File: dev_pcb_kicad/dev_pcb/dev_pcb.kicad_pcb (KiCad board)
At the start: 2 copper layers, 33 x 37.5 mm, 11 parts, among them U2 XIAO-ESP32-S3-DIP

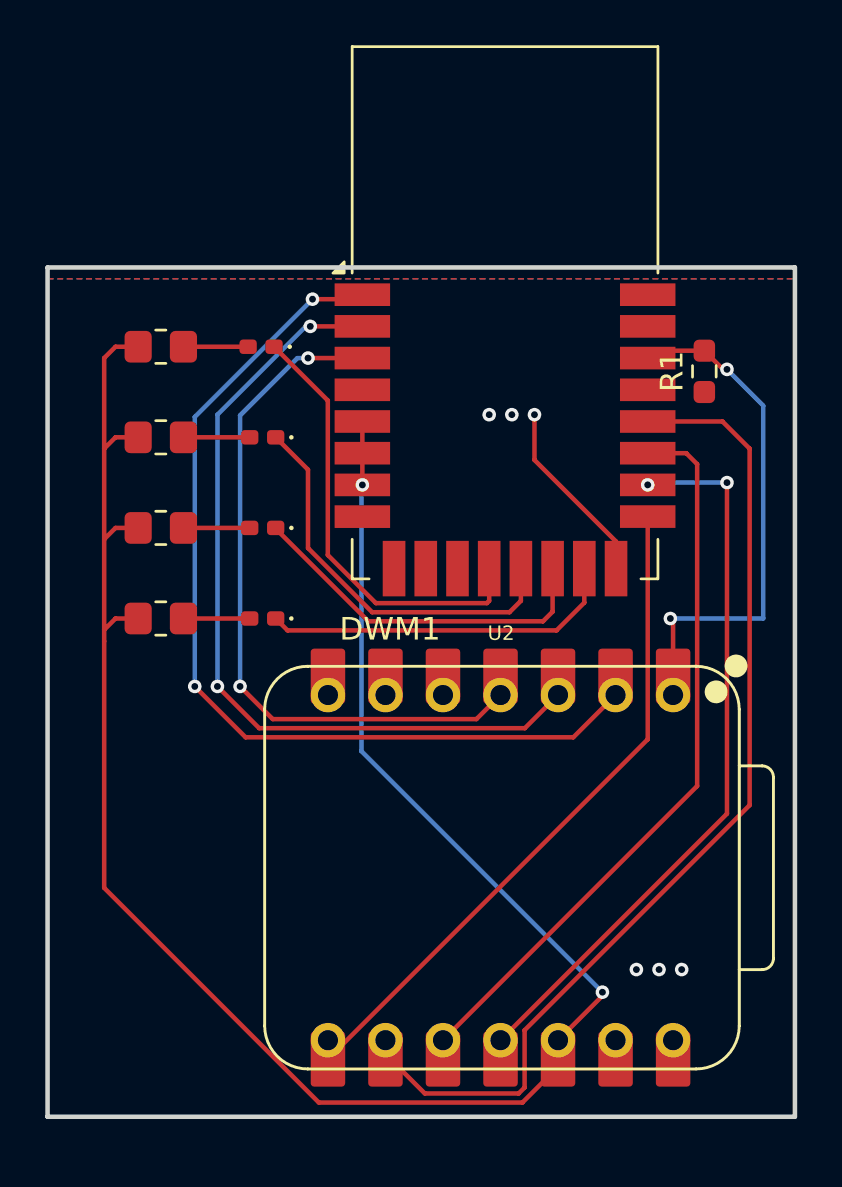
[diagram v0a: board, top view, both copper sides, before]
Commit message: .
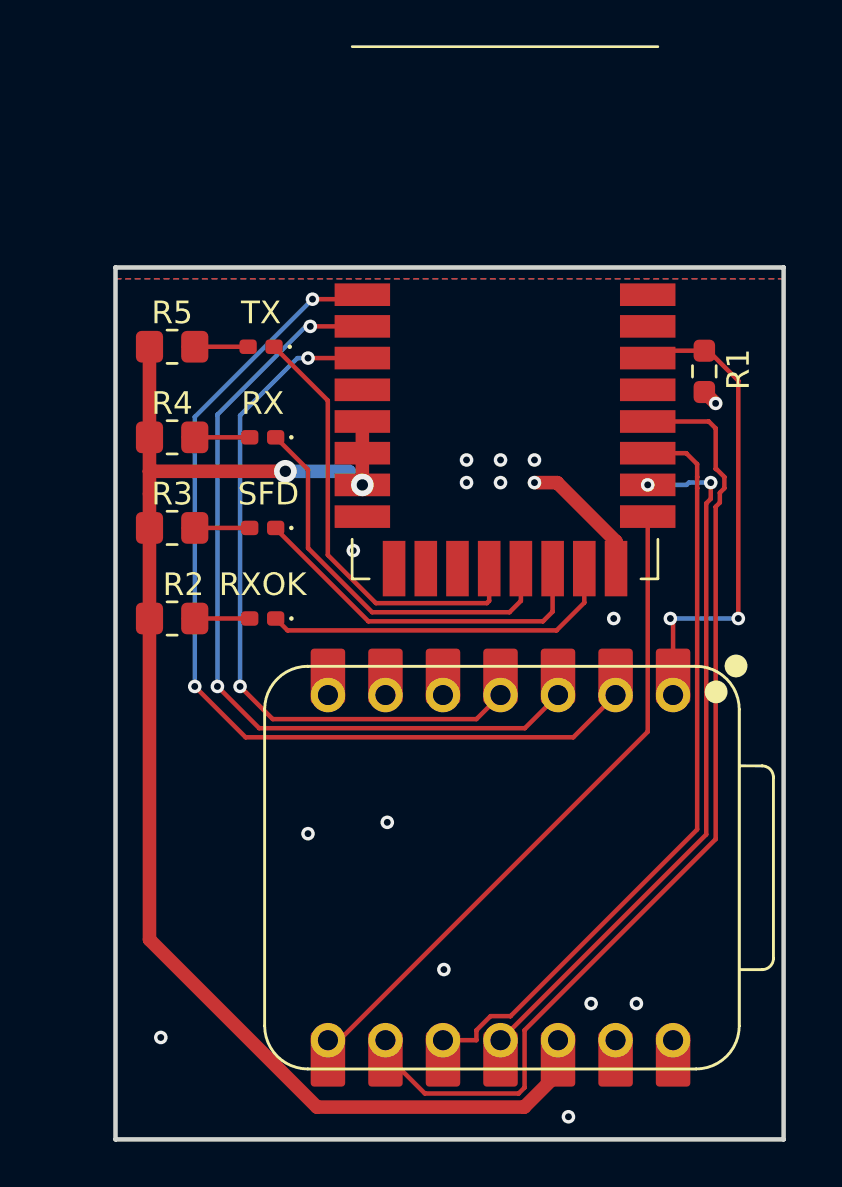
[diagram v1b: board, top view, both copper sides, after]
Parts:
- moved R2 0.50 mm to (70.5, 87.0)
- moved R3 0.50 mm to (70.5, 83.0)
- moved R4 0.50 mm to (70.5, 79.0)
- moved R5 0.50 mm to (70.5, 75.0)
- renumbered D3 to RX, D1 to RXOK, D2 to SFD, D4 to TX
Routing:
- net +3.3V: track 87.7 -> 61.0 mm
- net GND: track 8.29 -> 6.58 mm, vias 6 -> 16
- net Net-(DWM1-IRQ/GPIO8): track 23.2 -> 21.6 mm
- net Net-(DWM1-SPIMISO): track 32.5 -> 33.9 mm
- net Net-(DWM1-SPICLK): track 44.9 -> 43.6 mm
- net Net-(DWM1-SPIMOSI): track 32.3 -> 31.3 mm
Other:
- board size 33 x 37.5 mm -> 29.5 x 38.5 mm
